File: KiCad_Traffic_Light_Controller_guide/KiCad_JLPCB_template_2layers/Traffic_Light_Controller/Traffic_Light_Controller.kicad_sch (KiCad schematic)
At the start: 64 parts, among them J1 Conn_02x08_Odd_Even, J2 Conn_02x08_Odd_Even, J3 Conn_02x05_Odd_Even, J4 +5V, SW1 SW_Push, SW2 OVR, SW3 SW_SPDT, U1 SM420561N, U2 SM420561N, U3 LM1117DT-3.3

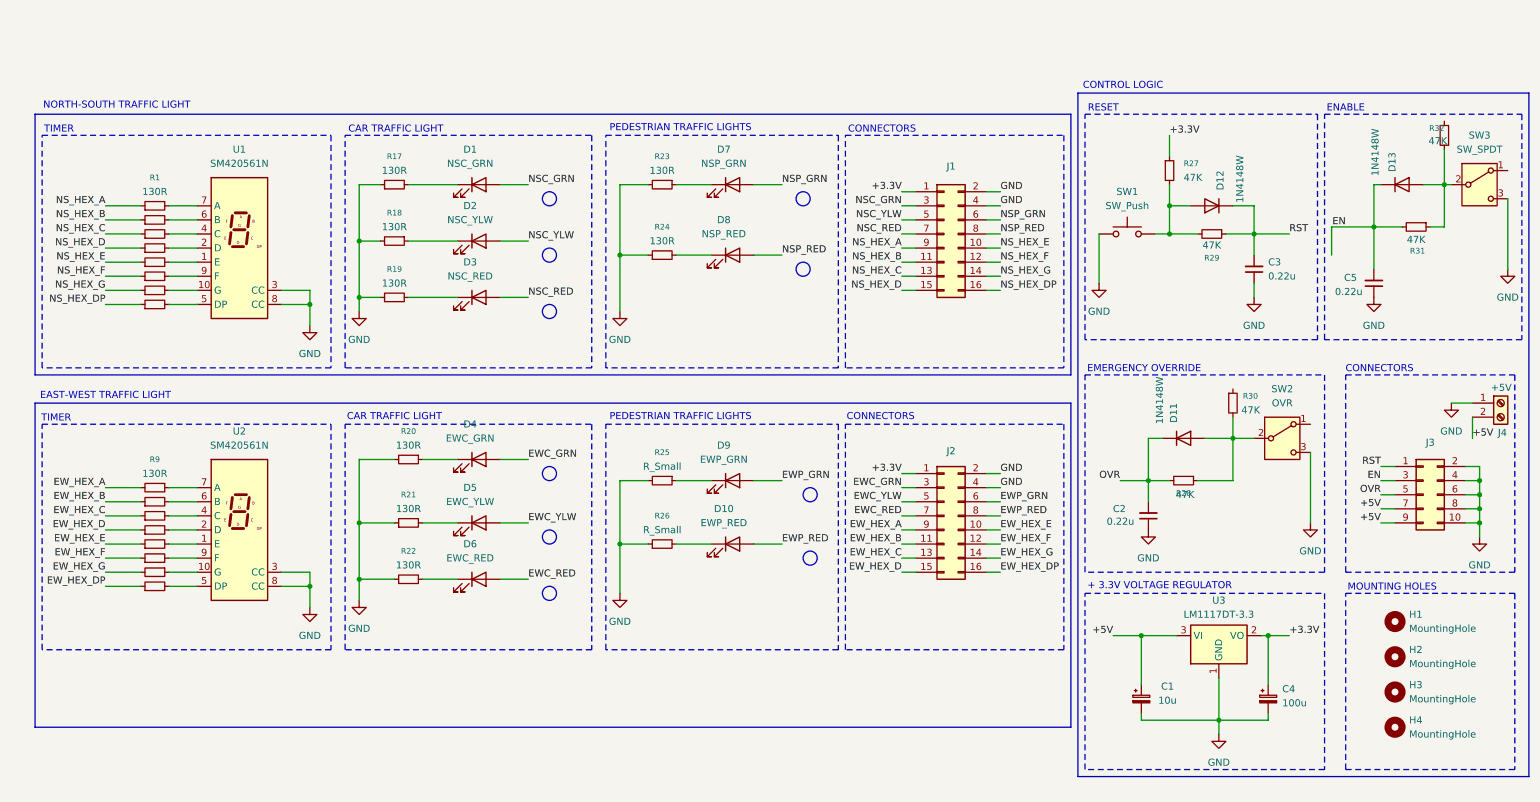
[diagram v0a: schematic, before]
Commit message: commit
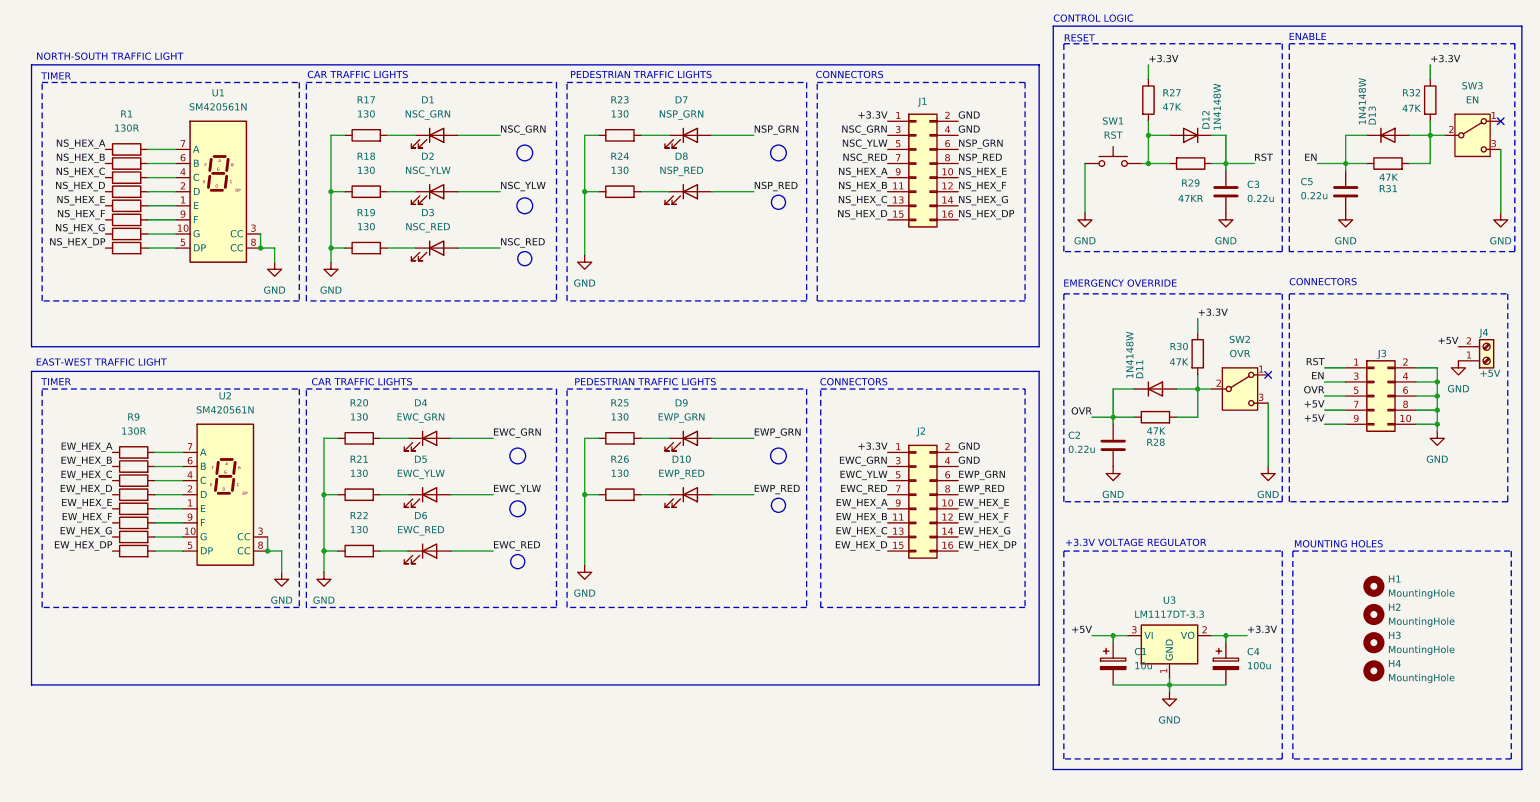
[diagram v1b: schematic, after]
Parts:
- removed C1: 10u, symbol Device:C_Polarized_Small
- removed C2, C3, C5: 0.22u, symbol Device:C_Small
- removed C4: 100u, symbol Device:C_Polarized_Small
- removed R1, R10, R11, R12, R13, R14, R15, R16, R17, R18, R19, R2, R20, R21, R22, R23, R24, R3, R4, R5, R6, R7, R8, R9: 130R, symbol Device:R_Small
- removed R25, R26: R_Small, symbol Device:R_Small
- removed R27, R28, R29, R30, R31, R32: 47K, symbol Device:R_Small
- added C1: 10u, Capacitor_SMD:CP_Elec_4x5.3, symbol Device:C_Polarized
- added C2, C3, C5: 0.22u, Capacitor_SMD:C_1206_3216Metric_Pad1.33x1.80mm_HandSolder, symbol Device:C
- added C4: 100u, Capacitor_SMD:CP_Elec_6.3x5.8, symbol Device:C_Polarized
- added R1, R9: 130R, Resistor_SMD:R_1206_3216Metric_Pad1.30x1.75mm_HandSolder, symbol Device:R
- added R10, R11, R12, R13, R14, R15, R16, R2, R3, R4, R5, R6, R7, R8: R, Resistor_SMD:R_1206_3216Metric_Pad1.30x1.75mm_HandSolder, symbol Device:R
- added R17, R18, R19, R20, R21, R22, R23, R24, R25, R26: 130, Resistor_SMD:R_1206_3216Metric_Pad1.30x1.75mm_HandSolder, symbol Device:R
- added R27, R28, R30, R31, R32: 47K, Resistor_SMD:R_1206_3216Metric_Pad1.30x1.75mm_HandSolder, symbol Device:R
- added R29: 47KR, Resistor_SMD:R_1206_3216Metric_Pad1.30x1.75mm_HandSolder, symbol Device:R
- D1, D10, D2, D3, D4, D5, D6, D7, D8, D9: footprint (none) -> LED_THT:LED_D5.0mm
- H1, H2, H3, H4: footprint (none) -> MountingHole:MountingHole_2.2mm_M2
- J1, J2: footprint (none) -> Connector_PinHeader_2.54mm:PinHeader_2x08_P2.54mm_Vertical
- J3: footprint (none) -> Connector_PinHeader_2.54mm:PinHeader_2x05_P2.54mm_Vertical
- J4: footprint (none) -> my_footprints:Terminal_Block_5mm
- SW1: value SW_Push -> RST; footprint (none) -> my_footprints:tact_switch_5mm
- SW2: footprint (none) -> my_footprints:slide_switch_2.54mm
- SW3: value SW_SPDT -> EN; footprint (none) -> my_footprints:slide_switch_2.54mm
- U3: footprint Package_TO_SOT_SMD:TO-252-3_TabPin2 -> Package_TO_SOT_SMD:SOT-223-3_TabPin2
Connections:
- net +3.3V: now also C4.1, R27.1, R30.1, R32.1
- net +5V: now also C1.1
- net EN: now also C5.1, R31.1
- net EW_HEX_A: now also R9.1
- net EW_HEX_B: now also R10.1
- net EW_HEX_C: now also R11.1
- net EW_HEX_D: now also R12.1
- net EW_HEX_DP: now also R16.1
- net EW_HEX_E: now also R13.1
- net EW_HEX_F: now also R14.1
- net EW_HEX_G: now also R15.1
- net GND: now also C1.2, C2.2, C3.2, C4.2, C5.2, R17.1, R18.1, R19.1, R20.1, R21.1, R22.1, R23.1, R24.1, R25.1, R26.1
- net NS_HEX_A: now also R1.1
- net NS_HEX_B: now also R2.1
- net NS_HEX_C: now also R3.1
- net NS_HEX_D: now also R4.1
- net NS_HEX_DP: now also R8.1
- net NS_HEX_E: now also R5.1
- net NS_HEX_F: now also R6.1
- net NS_HEX_G: now also R7.1
- net OVR: now also C2.1, R28.1
- net RST: now also C3.1, R29.1
- net at D6.1 (K): now also R22.2
- net at U1.4 (C): now also R3.2
- net at U2.4 (C): now also R11.2
- net at D13.2 (A), SW3.2 (B): now also R31.2, R32.2
- net at D12.2 (A), SW1.2: now also R27.2, R29.2
- net at D11.2 (A), SW2.2 (B): now also R28.2, R30.2
- net at D5.1 (K): now also R21.2
- net at U1.1 (E): now also R5.2
- net at U1.10 (G): now also R7.2
- net at U1.2 (D): now also R4.2
- net at U1.5 (DP): now also R8.2
- net at U1.6 (B): now also R2.2
- net at U1.7 (A): now also R1.2
- net at U1.9 (F): now also R6.2
- net at U2.1 (E): now also R13.2
- net at D1.1 (K): now also R17.2
- net at D4.1 (K): now also R20.2
- net at D9.1 (K): now also R25.2
- net at D3.1 (K): now also R19.2
- net at U2.9 (F): now also R14.2
- net at D8.1 (K): now also R24.2
- net at U2.5 (DP): now also R16.2
- net at D7.1 (K): now also R23.2
- net at U2.10 (G): now also R15.2
- net at U2.2 (D): now also R12.2
- net at U2.6 (B): now also R10.2
- net at U2.7 (A): now also R9.2
- net at D2.1 (K): now also R18.2
- net at D10.1 (K): now also R26.2
- no-connect marks 0 -> 2
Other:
- note added: "+3.3V VOLTAGE REGULATOR"
- note added: "CAR TRAFFIC LIGHTS"
- note removed: "+ 3.3V VOLTAGE REGULATOR"
- note removed: "CAR TRAFFIC LIGHT"

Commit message: KICAD 9
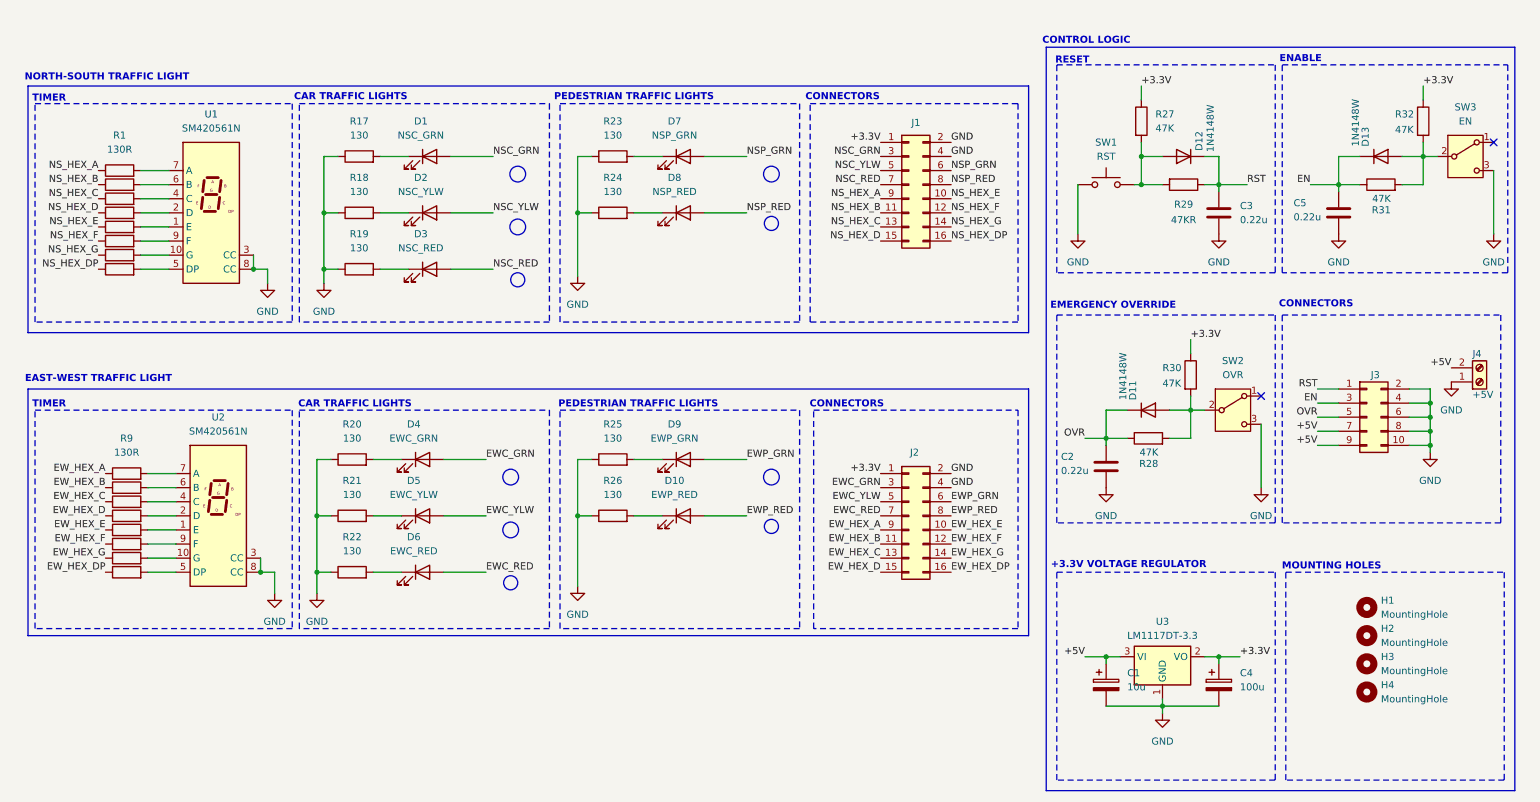
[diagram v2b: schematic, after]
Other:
- moved on the sheet: C1, C2, C3, C4, C5, D1, D10, D11, D12, D13, D2, D3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
